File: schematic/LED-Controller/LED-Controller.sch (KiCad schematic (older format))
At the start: 14 parts, among them J1 5V Power, J2 ICSP, J3 RCin, J4 Serial Connect, J5 TSW-102-08-L-T-RA, J6 TSW-102-08-L-T-RA, J7 TSW-102-08-L-T-RA, U1 PIC18F27Q43-xSO

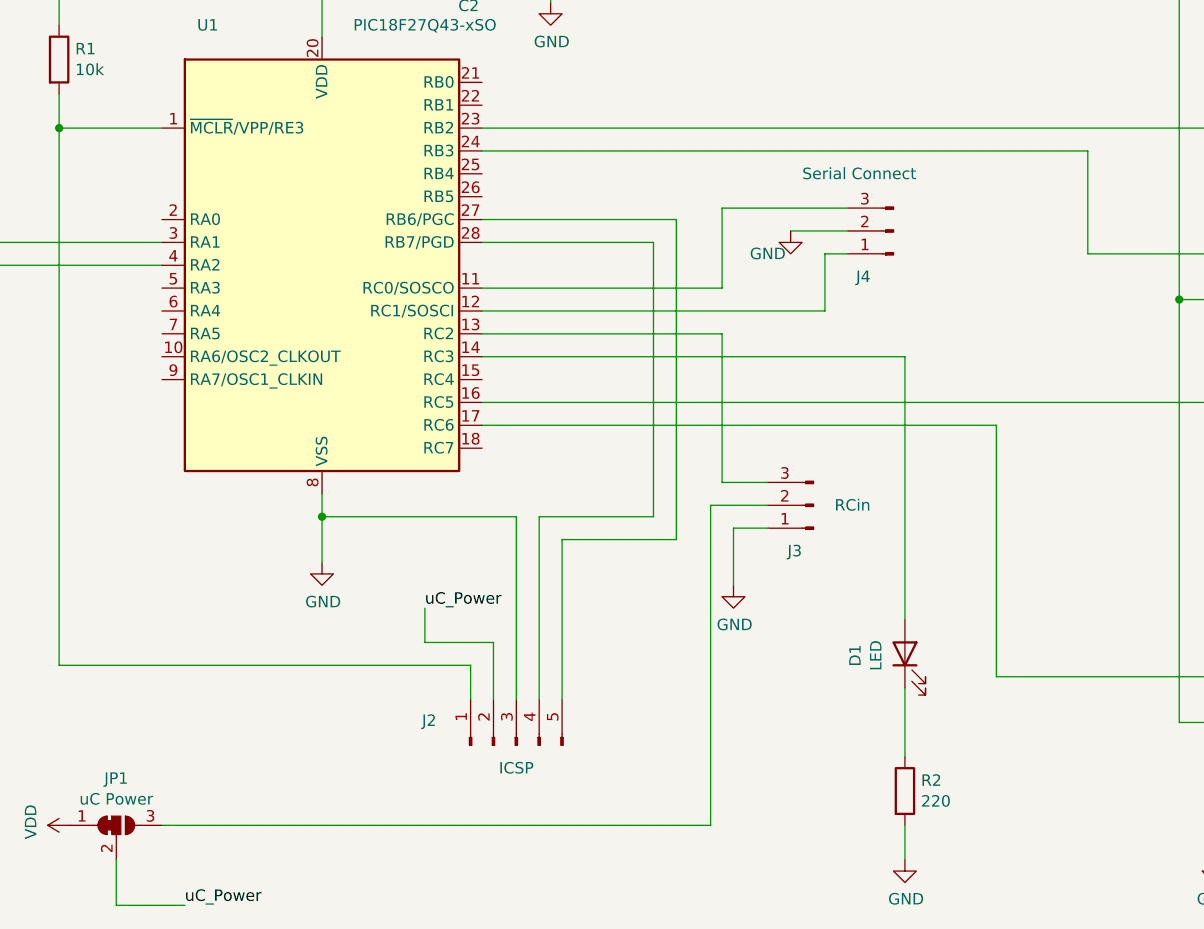
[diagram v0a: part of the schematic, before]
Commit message: Complete pcb layout
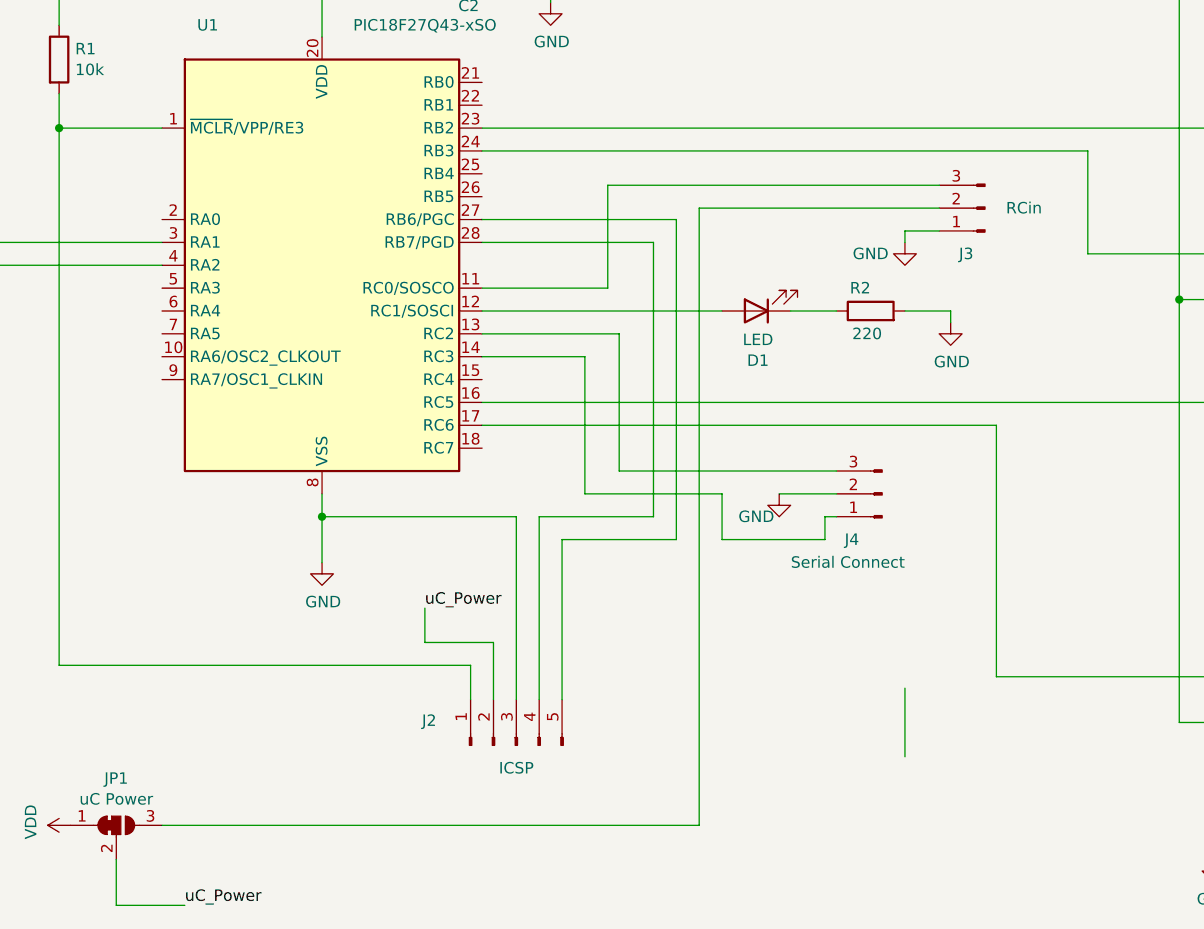
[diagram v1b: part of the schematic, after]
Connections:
- net at J3.3 (Pin_3): now also U1.11 (RC0/SOSCO); no longer U1.13 (RC2)
- net at J4.1 (Pin_1): now also U1.14 (RC3); no longer U1.12 (RC1/SOSCI)
- net at J4.3 (Pin_3): now also U1.13 (RC2); no longer U1.11 (RC0/SOSCO)
- net at D1.2 (A): now also U1.12 (RC1/SOSCI); no longer U1.14 (RC3)
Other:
- moved on the sheet: D1, J3, J4, R2
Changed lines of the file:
@@
 L Connector:Conn_01x03_Male J4
 U 1 1 602A7478
-P 6950 3400
-F 0 "J4" H 7050 3600 50  0000 L CNN
-F 1 "Serial Connect" H 6850 3150 50  0000 L CNN
-F 2 "Connector_PinHeader_2.54mm:PinHeader_1x03_P2.54mm_Vertical" H 6950 3400 50  0001 C CNN
-F 3 "~" H 6950 3400 50  0001 C CNN
-	1    6950 3400
+P 6900 4550
+F 0 "J4" H 7000 4750 50  0000 L CNN
+F 1 "Serial Connect" H 6800 4850 50  0000 L CNN
+F 2 "Connector_PinHeader_2.54mm:PinHeader_1x03_P2.54mm_Vertical" H 6900 4550 50  0001 C CNN
+F 3 "~" H 6900 4550 50  0001 C CNN
+	1    6900 4550
 	-1   0    0    1
 $EndComp
@@
 L Connector:Conn_01x03_Male J3
 U 1 1 6029D4DE
-P 6600 4600
-F 0 "J3" H 6650 4800 50  0000 L CNN
-F 1 "RCin" H 6350 4600 50  0000 L CNN
-F 2 "Connector_PinHeader_2.54mm:PinHeader_1x03_P2.54mm_Horizontal" H 6600 4600 50  0001 C CNN
-F 3 "~" H 6600 4600 50  0001 C CNN
-	1    6600 4600
+P 7350 3300
+F 0 "J3" H 7400 3500 50  0000 L CNN
+F 1 "RCin" H 7100 3300 50  0000 L CNN
+F 2 "Connector_PinHeader_2.54mm:PinHeader_1x03_P2.54mm_Horizontal" H 7350 3300 50  0001 C CNN
+F 3 "~" H 7350 3300 50  0001 C CNN
+	1    7350 3300
 	-1   0    0    1
 $EndComp
@@
 Wire Wire Line
 	2750 3550 2750 1500
-Wire Wire Line
-	6650 3500 6750 3500
-Wire Wire Line
-	5150 3650 6200 3650
-$Comp
-L power:GND #PWR07
-U 1 1 602BC9A3
-P 6500 3400
-F 0 "#PWR07" H 6500 3150 50  0001 C CNN
-F 1 "GND" H 6400 3300 50  0000 C CNN
-F 2 "" H 6500 3400 50  0001 C CNN
-F 3 "" H 6500 3400 50  0001 C CNN
-	1    6500 3400
-	1    0    0    -1
-$EndComp
-Wire Wire Line
-	6750 3400 6500 3400
-Wire Wire Line
-	5150 3850 6200 3850
-Wire Wire Line
-	6200 3850 6200 4500
-Wire Wire Line
-	6200 4500 6400 4500
 $Comp
 L power:GND #PWR06
 U 1 1 602C1BEB
-P 6250 4950
-F 0 "#PWR06" H 6250 4700 50  0001 C CNN
-F 1 "GND" H 6255 4777 50  0000 C CNN
-F 2 "" H 6250 4950 50  0001 C CNN
-F 3 "" H 6250 4950 50  0001 C CNN
-	1    6250 4950
-	1    0    0    -1
-$EndComp
-Wire Wire Line
-	6400 4700 6250 4700
-Wire Wire Line
-	6250 4700 6250 4950
+P 7000 3450
+F 0 "#PWR06" H 7000 3200 50  0001 C CNN
+F 1 "GND" H 6850 3400 50  0000 C CNN
+F 2 "" H 7000 3450 50  0001 C CNN
+F 3 "" H 7000 3450 50  0001 C CNN
+	1    7000 3450
+	1    0    0    -1
+$EndComp
+Wire Wire Line
+	7150 3400 7000 3400
+Wire Wire Line
+	7000 3400 7000 3450
 $Comp
 L Device:LED D1
 U 1 1 602B6ED3
-P 7000 5250
-F 0 "D1" H 6993 5467 50  0000 C CNN
-F 1 "LED" H 6993 5376 50  0000 C CNN
-F 2 "LED_SMD:LED_0603_1608Metric_Pad1.05x0.95mm_HandSolder" H 7000 5250 50  0001 C CNN
-F 3 "~" H 7000 5250 50  0001 C CNN
-	1    7000 5250
-	0    -1   -1   0
+P 6350 3750
+F 0 "D1" H 6343 3967 50  0000 C CNN
+F 1 "LED" H 6343 3876 50  0000 C CNN
+F 2 "LED_SMD:LED_0603_1608Metric_Pad1.05x0.95mm_HandSolder" H 6350 3750 50  0001 C CNN
+F 3 "~" H 6350 3750 50  0001 C CNN
+	1    6350 3750
+	-1   0    0    1
 $EndComp
 $Comp
 L Device:R R2
 U 1 1 602B7BC0
-P 7000 5850
-F 0 "R2" H 7070 5896 50  0000 L CNN
-F 1 "220" H 7070 5805 50  0000 L CNN
-F 2 "Resistor_SMD:R_0603_1608Metric" V 6930 5850 50  0001 C CNN
-F 3 "~" H 7000 5850 50  0001 C CNN
-	1    7000 5850
-	1    0    0    -1
-$EndComp
-$Comp
-L power:GND #PWR08
-U 1 1 602B7F4F
-P 7000 6150
-F 0 "#PWR08" H 7000 5900 50  0001 C CNN
-F 1 "GND" H 7005 5977 50  0000 C CNN
-F 2 "" H 7000 6150 50  0001 C CNN
-F 3 "" H 7000 6150 50  0001 C CNN
-	1    7000 6150
-	1    0    0    -1
-$EndComp
-Wire Wire Line
-	7000 6150 7000 6000
-Wire Wire Line
-	5150 3950 7000 3950
-Wire Wire Line
-	7000 3950 7000 5100
+P 6850 3750
+F 0 "R2" V 6950 3750 50  0000 L CNN
+F 1 "220" V 6750 3700 50  0000 L CNN
+F 2 "Resistor_SMD:R_0603_1608Metric" V 6780 3750 50  0001 C CNN
+F 3 "~" H 6850 3750 50  0001 C CNN
+	1    6850 3750
+	0    -1   -1   0
+$EndComp
 Wire Wire Line
 	7000 5400 7000 5700
@@
 Wire Wire Line
 	4450 2300 4850 2300
-Wire Wire Line
-	6650 3750 6650 3500
-Wire Wire Line
-	6200 3300 6200 3650
-Wire Wire Line
-	6200 3300 6750 3300
-Wire Wire Line
-	5150 3750 6650 3750
 Text Label 4450 2000 0    50   ~ 0
 uC_Power
@@
 	4450 2300 4450 2000
 Wire Wire Line
-	6150 6000 6150 4600
-Wire Wire Line
-	6150 4600 6400 4600
-Wire Wire Line
-	3750 6000 6150 6000
+	3750 6000 6100 6000
 Wire Wire Line
 	5100 5450 5100 5300
@@
 	5150 4250 7400 4250
 Wire Wire Line
-	5150 4150 9550 4150
-Wire Wire Line
 	9550 4150 9550 5450
 Wire Wire Line
@@
 Wire Wire Line
 	9550 2950 9550 3600
+$Comp
+L power:GND #PWR08
+U 1 1 602B7F4F
+P 7200 3800
+F 0 "#PWR08" H 7200 3550 50  0001 C CNN
+F 1 "GND" H 7205 3627 50  0000 C CNN
+F 2 "" H 7200 3800 50  0001 C CNN
+F 3 "" H 7200 3800 50  0001 C CNN
+	1    7200 3800
+	1    0    0    -1
+$EndComp
+Wire Wire Line
+	6500 3750 6700 3750
+Wire Wire Line
+	7000 3750 7200 3750
+Wire Wire Line
+	7200 3750 7200 3800
+Wire Wire Line
+	5150 3650 5700 3650
+Wire Wire Line
+	5700 3650 5700 3200
+Wire Wire Line
+	5700 3200 7150 3200
+Wire Wire Line
+	5150 3750 6200 3750
+Wire Wire Line
+	6700 4550 6450 4550
+$Comp
+L power:GND #PWR07
+U 1 1 602BC9A3
+P 6450 4550
+F 0 "#PWR07" H 6450 4300 50  0001 C CNN
+F 1 "GND" H 6350 4450 50  0000 C CNN
+F 2 "" H 6450 4550 50  0001 C CNN
+F 3 "" H 6450 4550 50  0001 C CNN
+	1    6450 4550
+	1    0    0    -1
+$EndComp
+Wire Wire Line
+	5150 3850 5750 3850
+Wire Wire Line
+	5750 3850 5750 4450
+Wire Wire Line
+	5750 4450 6700 4450
+Wire Wire Line
+	5150 4150 9550 4150
+Wire Wire Line
+	5150 3950 5600 3950
+Wire Wire Line
+	5600 3950 5600 4550
+Wire Wire Line
+	5600 4550 6200 4550
+Wire Wire Line
+	6200 4550 6200 4750
+Wire Wire Line
+	6200 4750 6650 4750
+Wire Wire Line
+	6650 4750 6650 4650
+Wire Wire Line
+	6650 4650 6700 4650
+Wire Wire Line
+	7150 3300 6100 3300
+Wire Wire Line
+	6100 3300 6100 6000
 $EndSCHEMATC
